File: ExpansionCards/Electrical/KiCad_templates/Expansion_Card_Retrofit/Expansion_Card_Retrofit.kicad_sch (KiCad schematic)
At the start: 26 parts, among them J1 HDMI_A, P2 USB_C_Plug, U1 MS2130, U2 GD25D05CT, U3 USBLC6-2P6, Y1 Crystal

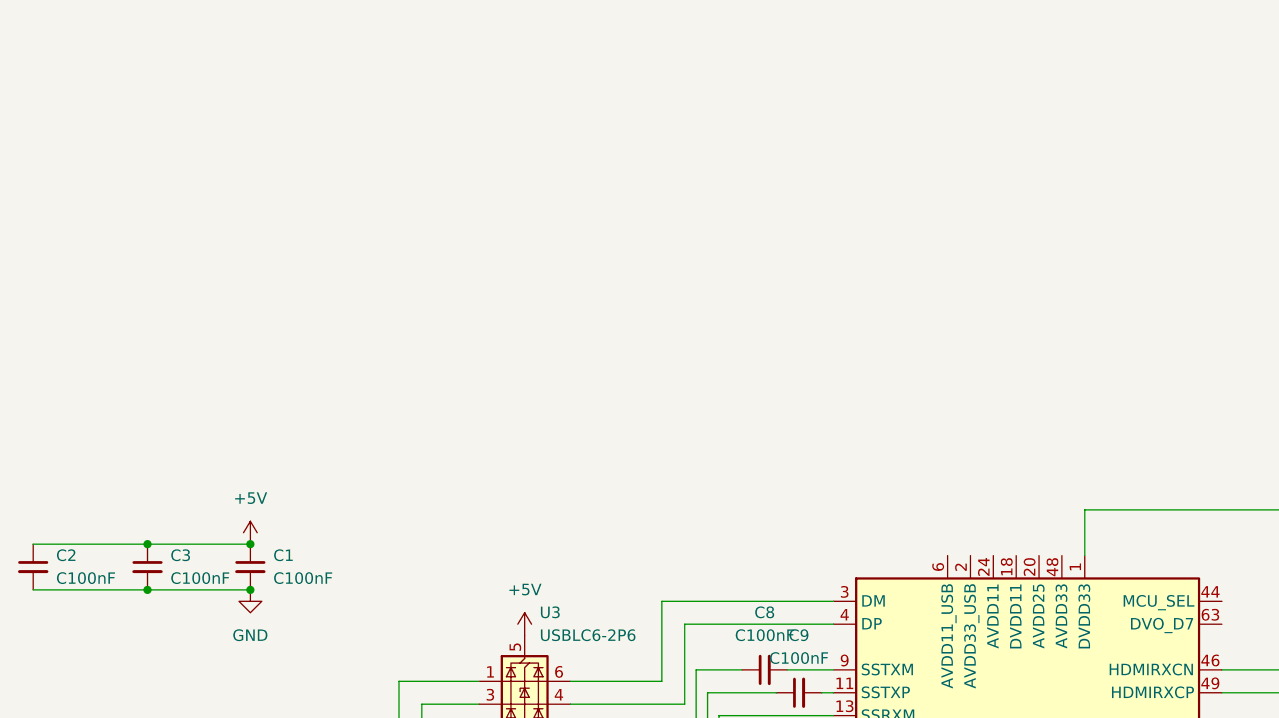
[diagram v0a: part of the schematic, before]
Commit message: Finished PCB design and add gerber files and BOM
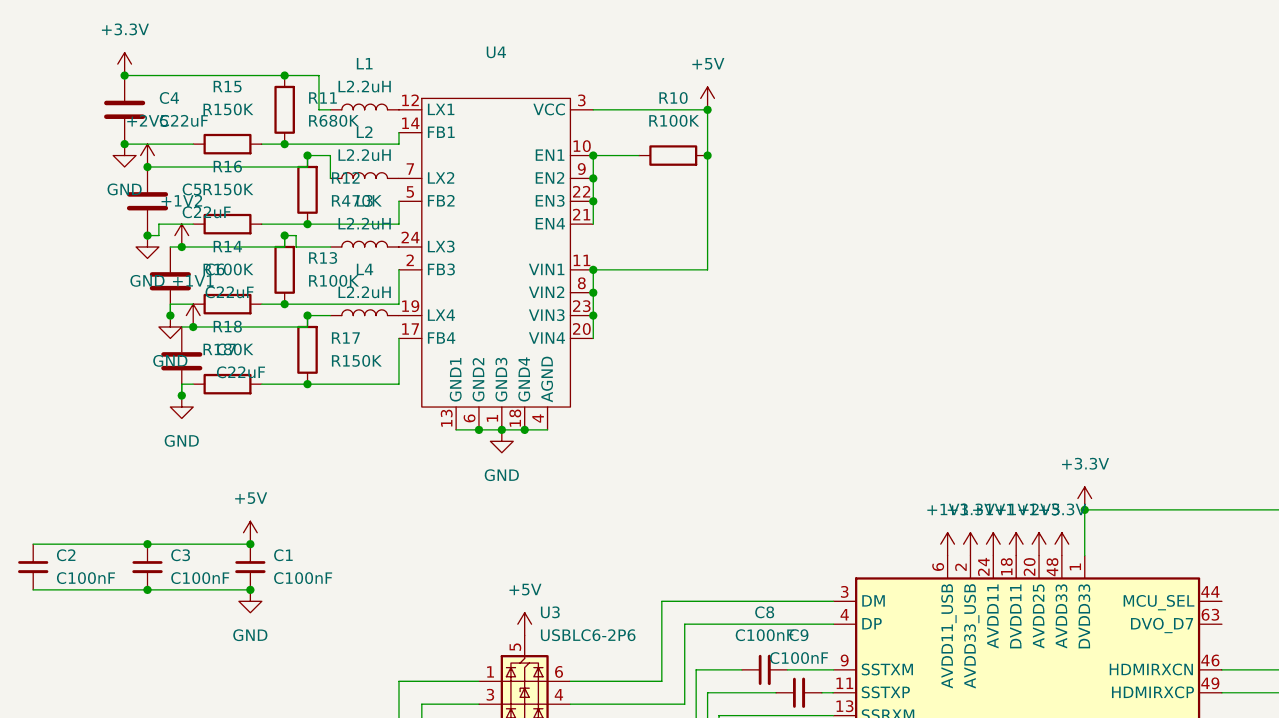
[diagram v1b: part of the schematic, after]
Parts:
- added C4, C5, C6, C7: C22uF, Capacitor_SMD:C_0201_0603Metric, symbol Device:C
- added L1, L2, L3, L4: L2.2uH, Inductor_SMD:L_0201_0603Metric, symbol Device:L
- added R10: R100K, Resistor_SMD:R_0201_0603Metric_Pad0.64x0.40mm_HandSolder, symbol Device:R
- added R11: R680K, Resistor_SMD:R_0201_0603Metric, symbol Device:R
- added R12: R470K, Resistor_SMD:R_0201_0603Metric, symbol Device:R
- added R13, R14: R100K, Resistor_SMD:R_0201_0603Metric, symbol Device:R
- added R15, R16, R17: R150K, Resistor_SMD:R_0201_0603Metric, symbol Device:R
- added R18: R180K, Resistor_SMD:R_0201_0603Metric, symbol Device:R
- added U4: ~, Package_DFN_QFN:HVQFN-24-1EP_4x4mm_P0.5mm_EP2.1x2.1mm, symbol EA3059_lib:EA3059
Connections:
- net +5V: now also R10.2, U4.11 (VIN1), U4.20 (VIN4), U4.23 (VIN3), U4.3 (VCC), U4.8 (VIN2)
- net GND: now also C4.2, C5.2, C6.2, C7.2, R14.1, R15.1, R16.1, R18.1, U4.1 (GND3), U4.13 (GND1), U4.18 (GND4), U4.4 (AGND), U4.6 (GND2)
- net +3.3V: now reaches U1.1 (DVDD33), U1.16 (DVDD33), U1.31 (DVDD33), U1.33 (DVDD33), U1.41 (DVDD33), U2.3 (~{WP}), U2.8 (VCC)
- net +3.3V: now also U1.2 (AVDD33_USB), U1.48 (AVDD33), U1.5 (AVDD33_USB), U1.52 (AVDD33), U1.56 (AVDD33), U1.60 (AVDD33), U1.8 (AVDD33_USB), C4.1, L1.1, R11.2
- net +1V1: now reaches U1.10 (AVDD11_USB), U1.12 (AVDD11_USB), U1.6 (AVDD11_USB)
- net +1V1: now also U1.18 (DVDD11), U1.24 (AVDD11), U1.39 (DVDD11), U1.51 (AVDD11), U1.55 (AVDD11), U1.59 (AVDD11), C7.1, L4.1, R17.2
- net +2V5: now reaches U1.20 (AVDD25), U1.23 (AVDD25), U1.47 (AVDD25)
- net +2V5: now also C5.1, L2.1, R12.2
- new net: R13.1, R14.2, U4.2 (FB3)
- new net: R11.1, R15.2, U4.14 (FB1)
- new net: L1.2, U4.12 (LX1)
- new net: L3.2, U4.24 (LX3)
- new net: R17.1, R18.2, U4.17 (FB4)
- new net: R12.1, R16.2, U4.5 (FB2)
- new net: R10.1, U4.10 (EN1), U4.21 (EN4), U4.22 (EN3), U4.9 (EN2)
- new net: L4.2, U4.19 (LX4)
- new net: L2.2, U4.7 (LX2)
- new net +1V2: C6.1, L3.1, R13.2
